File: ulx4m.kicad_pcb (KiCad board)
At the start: 6 copper layers, 55.1 x 40 mm, 250 parts, among them J1 DF40C-100DP-0.4V(51), J2 DF40C-100DP-0.4V(51), J3 JTAG, U1 LFE5U-85F-6BG381C, U10 IS25LP128F-JBLE, U2 AS4C256M16D3, U3 TLV62569DBV, U4 TLV62569DBV, U5 TLV62569DBV, U6 TLV62569DBV, U8 KSZ9031RNXCA, U9 ASEMB-25.000MHZ-LC-T, Y1 FNETHE025

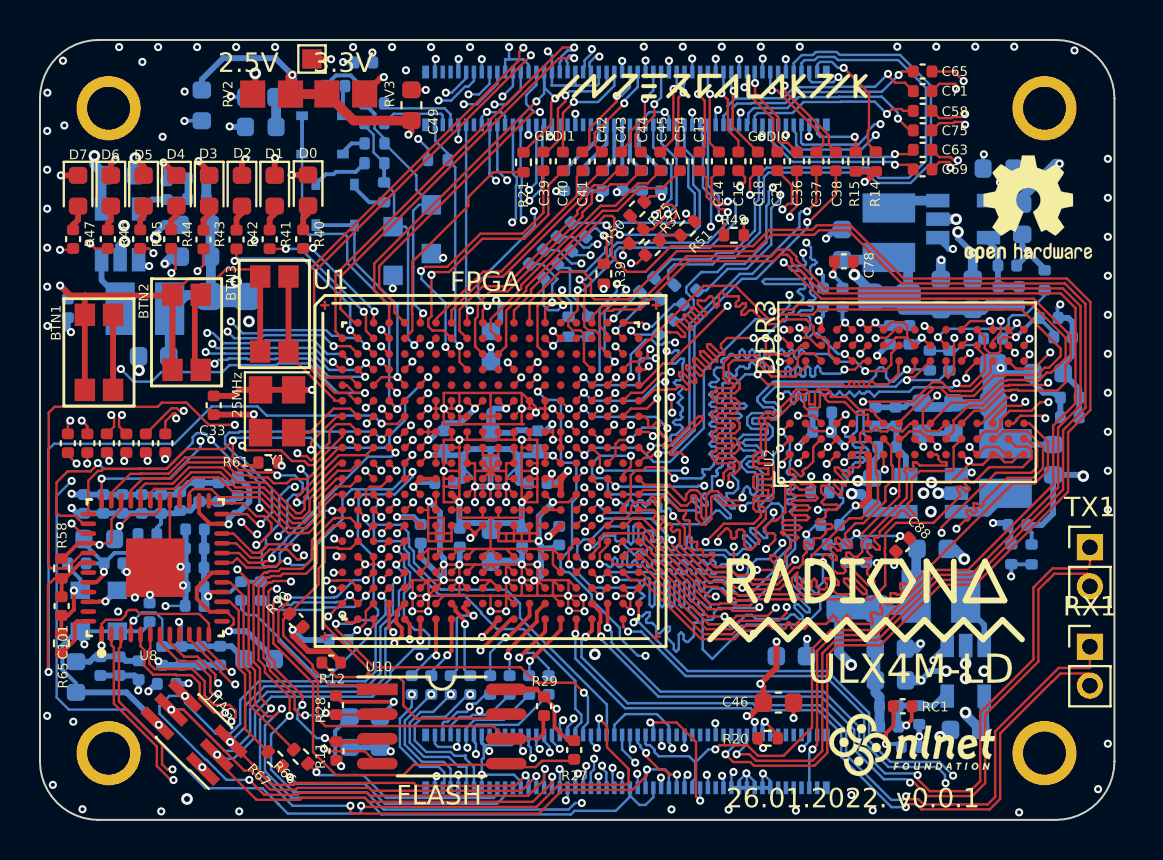
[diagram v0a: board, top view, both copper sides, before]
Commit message: Fix #17 DDR3 length matched - we should now be inside +-0.75mm
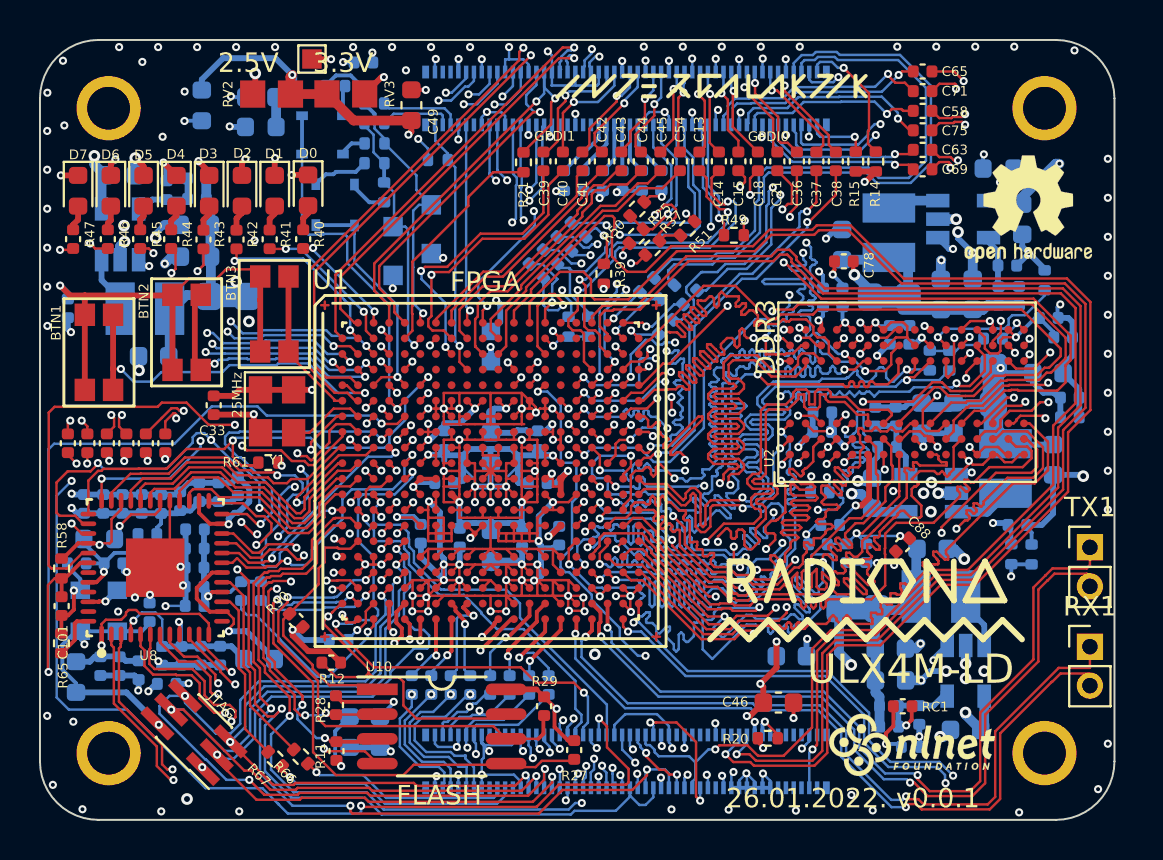
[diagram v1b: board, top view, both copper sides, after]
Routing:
- net DDR3_DQS1-: track 31.4 -> 35.0 mm
- net DDR3_DQ3: track 32.5 -> 35.5 mm
- net DDR3_DQ5: track 32.3 -> 35.1 mm
- net DDR3_DQ7: track 32.3 -> 35.0 mm
- net DDR3_ODT: track 32.8 -> 35.3 mm
- net DDR3_DQS1+: track 32.7 -> 35.0 mm
- net DDR3_DQ9: track 32.7 -> 35.0 mm
- net DDR3_DQ11: track 32.8 -> 35.0 mm
- net DDR3_DQ13: track 32.8 -> 35.0 mm
- net DDR3_A12: track 32.8 -> 35.0 mm
- net DDR3_DQ2: track 32.8 -> 35.0 mm
- net DDR3_DQ10: track 32.8 -> 34.9 mm
- net DDR3_A5: track 32.9 -> 35.0 mm
- net DDR3_A13: track 33.0 -> 35.0 mm
- net DDR3_A9: track 33.6 -> 35.6 mm
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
